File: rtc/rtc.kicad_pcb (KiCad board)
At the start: 2 copper layers, 40.4 x 36.5 mm, 14 parts, among them J1 Conn_02x03_Odd_Even, J2 Conn_01x04, J3 Conn_01x04, J4 Conn_01x04, U1 PCF8563T/5_518, Y1 LFXTAL016178REEL

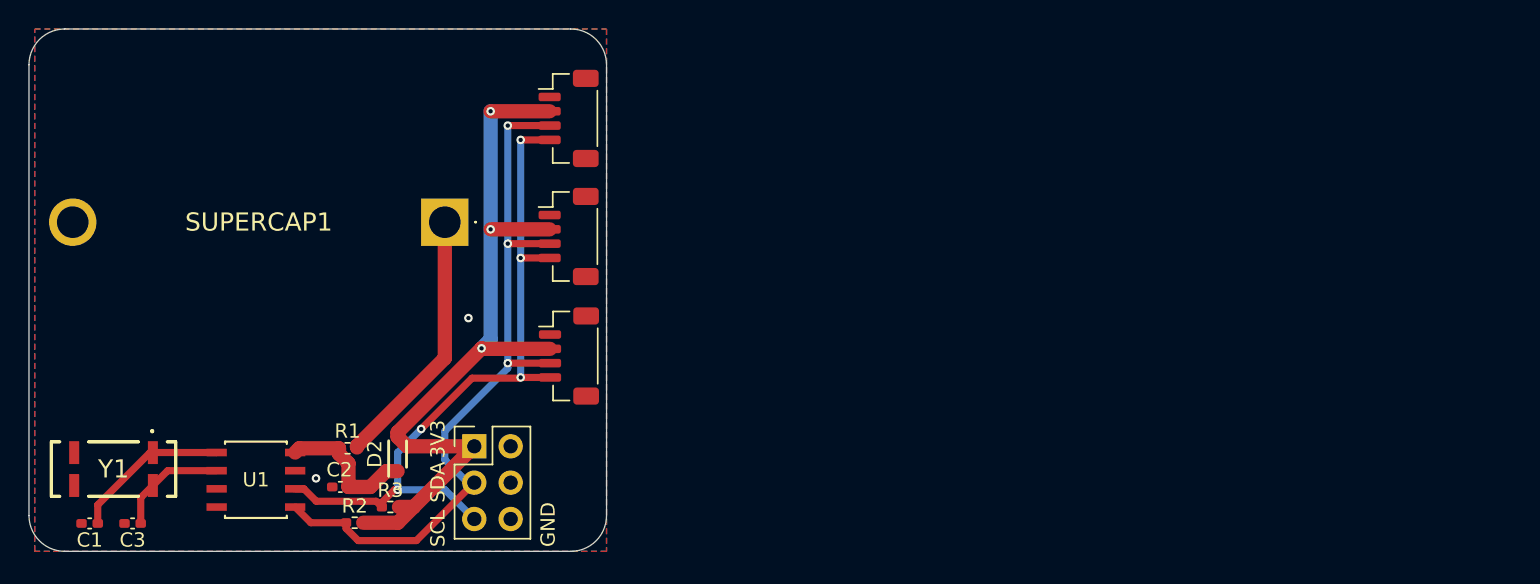
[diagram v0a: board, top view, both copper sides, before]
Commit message: rtc pcb iteration 2
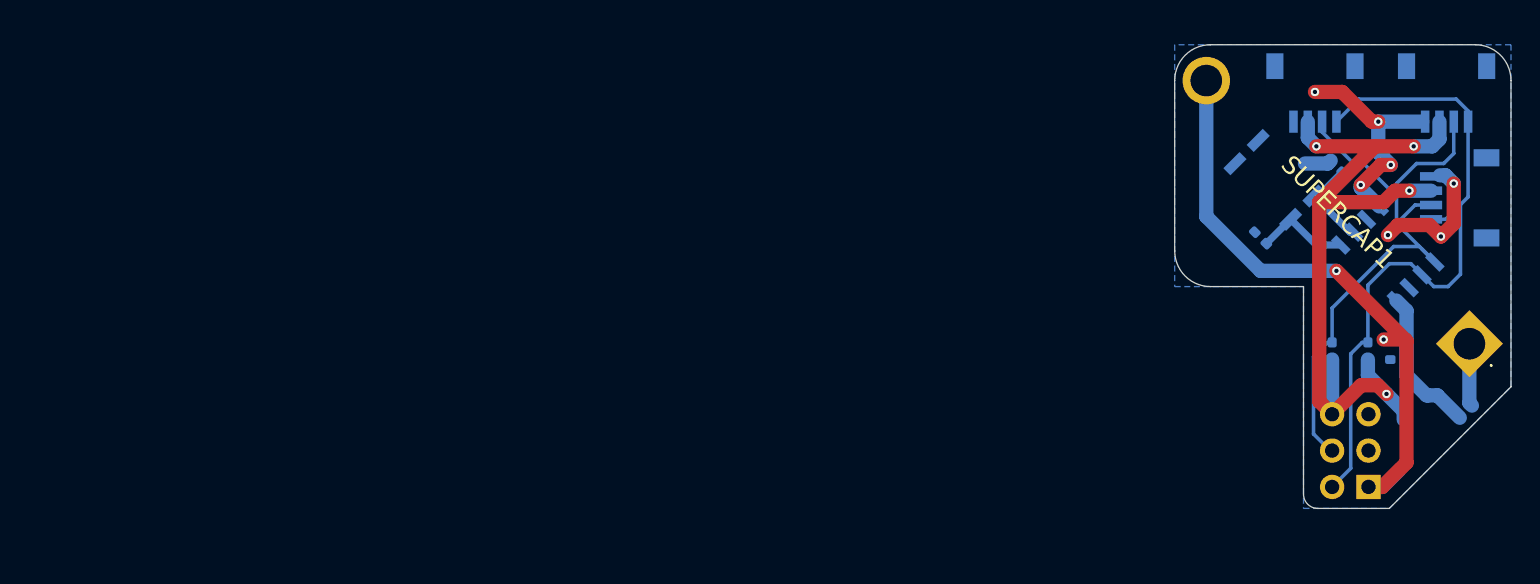
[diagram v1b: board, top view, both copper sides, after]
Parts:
- C1, C3: value C -> 24p; moved to B.Cu
- C2, D2, R1, R2, R3, U1, Y1: moved to B.Cu
- J1: footprint Connector_PinHeader_2.54mm:PinHeader_2x03_P2.54mm_Vertical -> Connector_PinSocket_2.54mm:PinSocket_2x03_P2.54mm_Vertical; moved to B.Cu
- J2, J3, J4: footprint pcb_footprints:JST_SH_BM04B-SRSS-TB_1x04-1MP_P1.00mm_Vertical -> pcb_footprints:SM04BSRSSTB; moved to B.Cu
- moved C3 87.7 mm to (152.3, 76.1), turned to 135 degrees
- moved C1 84.2 mm to (147.0, 81.1), turned to 135 degrees
- moved Y1 83.6 mm to (148.0, 77.0), turned to 135 degrees
- moved U1 80.7 mm to (155.9, 82.2), turned to -45 degrees
- moved R1 78.2 mm to (161.4, 93.3), turned to -135 degrees
- moved C2 74.5 mm to (156.6, 89.6)
- moved SUPERCAP1 72.1 mm to (161.6, 88.5), turned to -45 degrees
- moved D2 71.2 mm to (157.9, 92.9), turned to -135 degrees
- moved R2 69.3 mm to (152.0, 89.0), turned to -90 degrees
- moved R3 69.2 mm to (154.5, 89.0), turned to -90 degrees
- moved J2 64.1 mm to (160.0, 70.7), turned to 0 degrees
- moved J3 62.8 mm to (161.2, 78.3)
- moved J1 62.5 mm to (154.5, 98.5)
- moved J4 53.2 mm to (150.8, 70.7), turned to 0 degrees
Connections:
- J1 pad 1: +3.3V -> GND
- J1 pad 2: unconnected-(J1-Pin_2-Pad2) -> scl
- J1 pad 3: sda -> unconnected-(J1-Pin_3-Pad3)
- J1 pad 4: unconnected-(J1-Pin_4-Pad4) -> sda
- J1 pad 5: scl -> unconnected-(J1-Pin_5-Pad5)
- J1 pad 6: GND -> +3.3V
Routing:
- net GND: track 0.00 -> 71.1 mm, vias 2 -> 9
- net Net-(SUPERCAP1-+): track 18.3 -> 4.40 mm
- net sda: track 52.1 -> 44.9 mm, vias 3 -> 0
- net Net-(U1-OSCI): track 11.1 -> 6.65 mm
- net scl: track 50.6 -> 47.8 mm, vias 5 -> 0
- net Net-(U1-OSCO): track 7.89 -> 6.35 mm
- net +3.3V: track 55.1 -> 54.9 mm, vias 3 -> 4
- removed copper zone on F.Cu, net GND
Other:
- board size 40.4 x 36.5 mm -> 23.5 x 32.4 mm
- board text removed: "3V3"
- board text removed: "GND"
- board text removed: "SCL"
- board text removed: "SDA"
